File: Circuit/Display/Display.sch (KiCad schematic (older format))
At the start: 29 parts, among them J1 Conn_PIC_ICSP_ICD, J2 Conn_01x04_Female, U1 TBD62783A, U2 PIC16F18854-SO, U3 ULN2803A

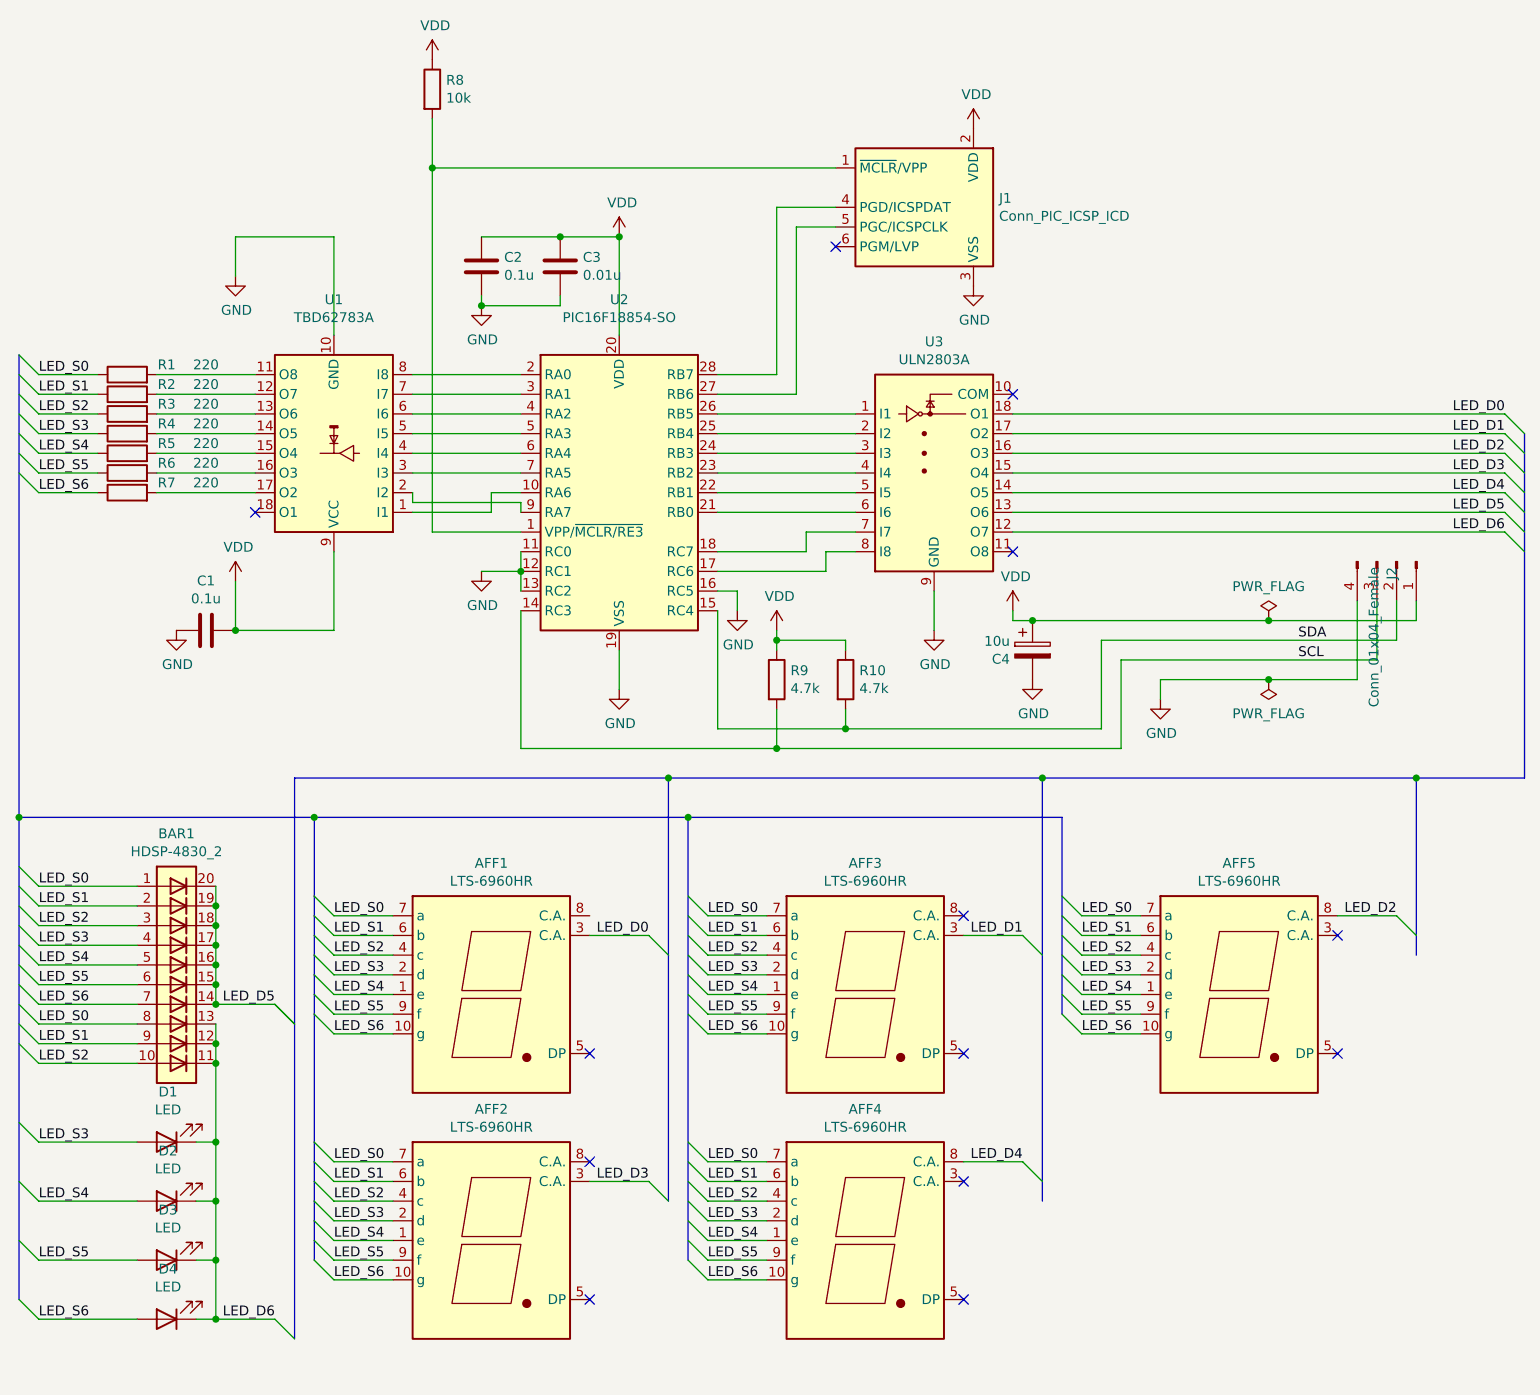
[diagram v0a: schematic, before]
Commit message: 回路完成
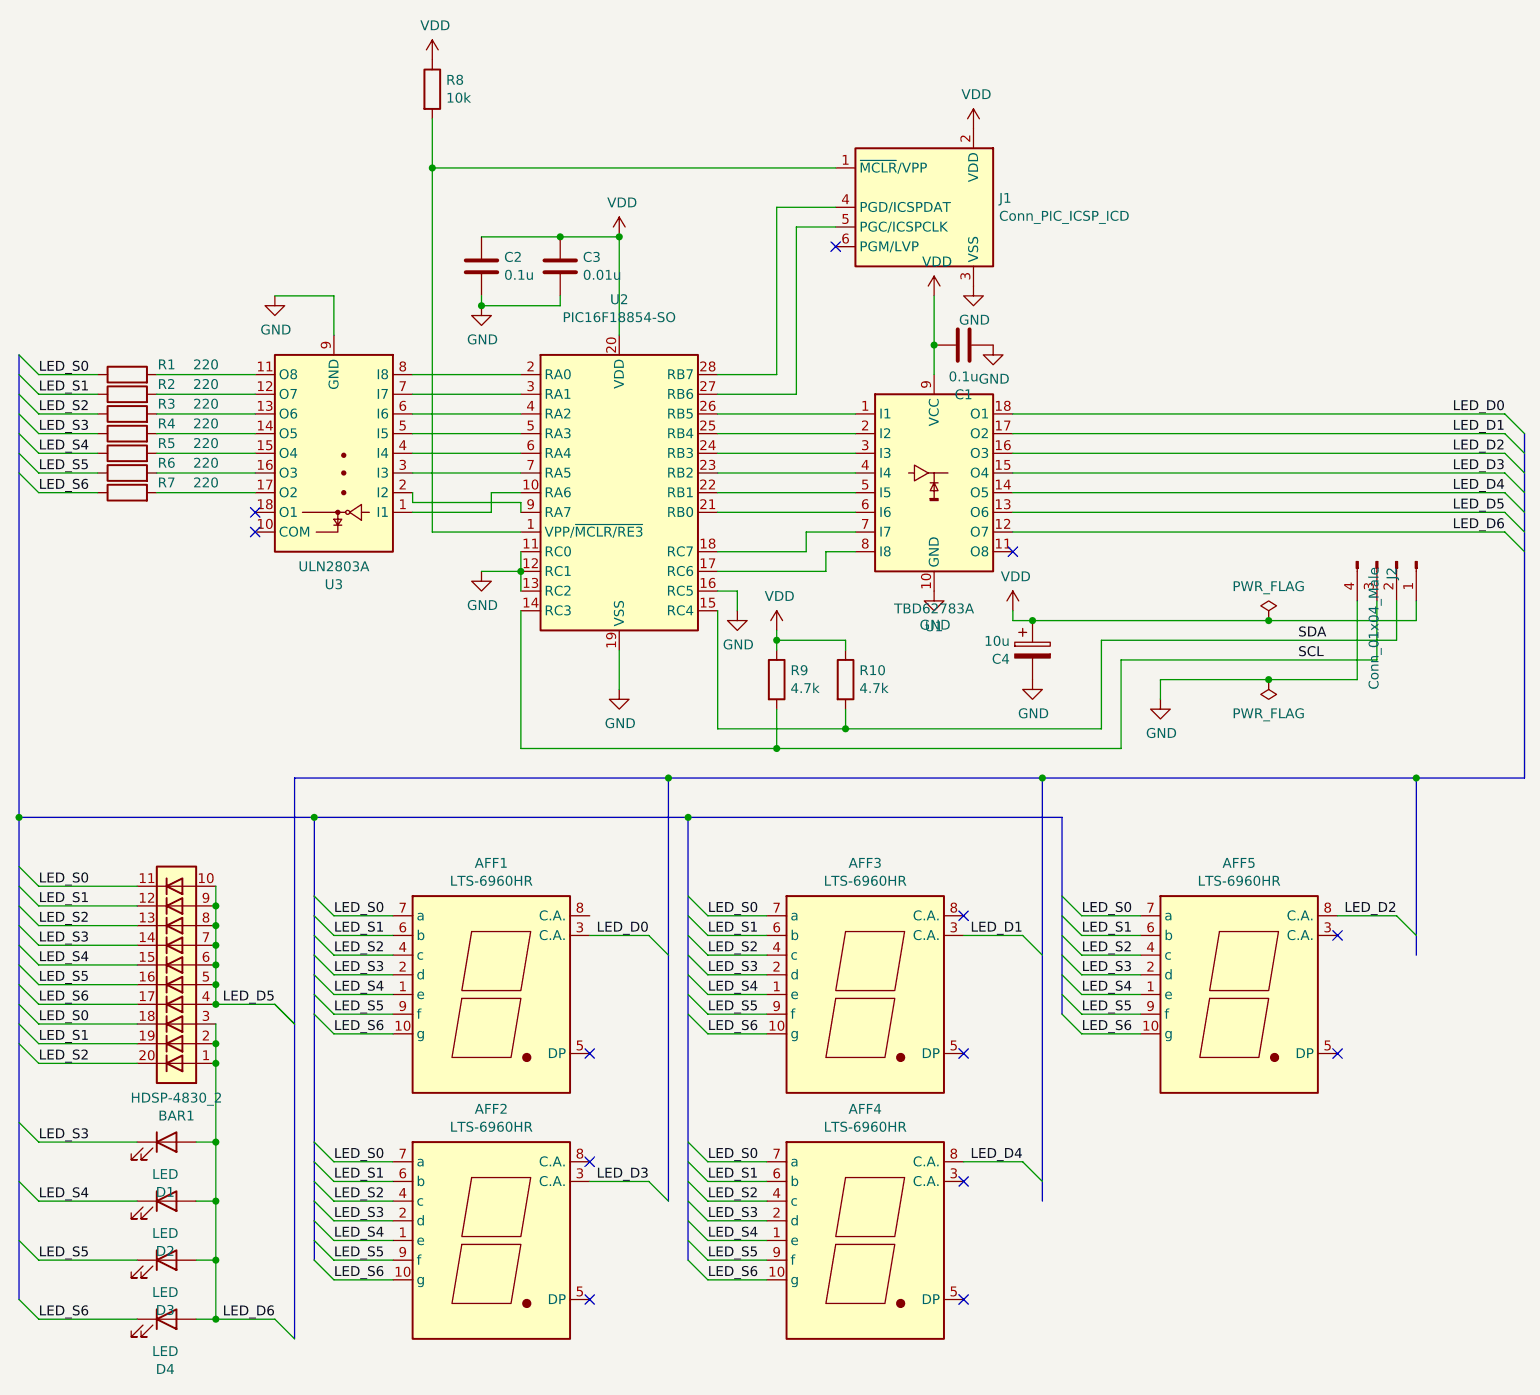
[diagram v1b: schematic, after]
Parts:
- J2: value Conn_01x04_Female -> Conn_01x04_Male
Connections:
- net LED_D0: now also U1.18 (O1); no longer U3.18 (O1)
- net LED_D1: now also U1.17 (O2); no longer U3.17 (O2)
- net LED_D2: now also U1.16 (O3); no longer U3.16 (O3)
- net LED_D3: now also U1.15 (O4); no longer U3.15 (O4)
- net LED_D4: now also U1.14 (O5); no longer U3.14 (O5)
- net LED_D5: now also BAR1.10 (A), BAR1.4 (A), BAR1.5 (A), BAR1.6 (A), BAR1.7 (A), BAR1.8 (A), BAR1.9 (A), U1.13 (O6); no longer BAR1.14 (K), BAR1.15 (K), BAR1.16 (K), BAR1.17 (K), BAR1.18 (K), BAR1.19 (K), BAR1.20 (K), U3.13 (O6)
- net LED_D6: now also BAR1.1 (A), BAR1.2 (A), BAR1.3 (A), D1.2 (A), D2.2 (A), D3.2 (A), D4.2 (A), U1.12 (O7); no longer BAR1.11 (K), BAR1.12 (K), BAR1.13 (K), D1.1 (K), D2.1 (K), D3.1 (K), D4.1 (K), U3.12 (O7)
- net LED_S0: now also BAR1.11 (K), BAR1.18 (K); no longer BAR1.1 (A), BAR1.8 (A)
- net LED_S1: now also BAR1.12 (K), BAR1.19 (K); no longer BAR1.2 (A), BAR1.9 (A)
- net LED_S2: now also BAR1.13 (K), BAR1.20 (K); no longer BAR1.10 (A), BAR1.3 (A)
- net LED_S3: now also BAR1.14 (K), D1.1 (K); no longer BAR1.4 (A), D1.2 (A)
- net LED_S4: now also BAR1.15 (K), D2.1 (K); no longer BAR1.5 (A), D2.2 (A)
- net LED_S5: now also BAR1.16 (K), D3.1 (K); no longer BAR1.6 (A), D3.2 (A)
- net LED_S6: now also BAR1.17 (K), D4.1 (K); no longer BAR1.7 (A), D4.2 (A)
- net at U2.10 (RA6): now also U3.1 (I1); no longer U1.1 (I1)
- net at U2.17 (RC6): now also U1.8 (I8); no longer U3.8 (I8)
- net at U2.18 (RC7): now also U1.7 (I7); no longer U3.7 (I7)
- net at U2.2 (RA0): now also U3.8 (I8); no longer U1.8 (I8)
- net at U2.21 (RB0): now also U1.6 (I6); no longer U3.6 (I6)
- net at U2.22 (RB1): now also U1.5 (I5); no longer U3.5 (I5)
- net at U2.23 (RB2): now also U1.4 (I4); no longer U3.4 (I4)
- net at U2.24 (RB3): now also U1.3 (I3); no longer U3.3 (I3)
- net at U2.25 (RB4): now also U1.2 (I2); no longer U3.2 (I2)
- net at U2.26 (RB5): now also U1.1 (I1); no longer U3.1 (I1)
- net at U2.3 (RA1): now also U3.7 (I7); no longer U1.7 (I7)
- net at U2.4 (RA2): now also U3.6 (I6); no longer U1.6 (I6)
- net at U2.5 (RA3): now also U3.5 (I5); no longer U1.5 (I5)
- net at U2.6 (RA4): now also U3.4 (I4); no longer U1.4 (I4)
- net at U2.7 (RA5): now also U3.3 (I3); no longer U1.3 (I3)
- net at U2.9 (RA7): now also U3.2 (I2); no longer U1.2 (I2)
- net at U1.11 (O8): no longer R1.2
- net at R2.2: now also U3.12 (O7); no longer U1.12 (O7)
- net at R3.2: now also U3.13 (O6); no longer U1.13 (O6)
- net at R4.2: now also U3.14 (O5); no longer U1.14 (O5)
- net at R5.2: now also U3.15 (O4); no longer U1.15 (O4)
- net at R6.2: now also U3.16 (O3); no longer U1.16 (O3)
- net at R7.2: now also U3.17 (O2); no longer U1.17 (O2)
- net at U3.11 (O8): now also R1.2
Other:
- moved on the sheet: C1, D1, D2, D3, D4, U1, U3
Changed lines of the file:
@@
 	4700 5900 5100 5900
 Wire Wire Line
-	4300 4500 3800 4500
-Wire Wire Line
-	4300 5000 4300 4500
-Wire Wire Line
-	4300 6500 4300 6100
-Wire Wire Line
-	3800 6500 4300 6500
+	7350 4800 7350 5050
 $Comp
 L Device:LED D4
@@
 F 3 "~" H 3450 10000 50  0001 C CNN
 	1    3450 10000
-	-1   0    0    1
+	1    0    0    -1
 $EndComp
 $Comp
@@
 F 3 "~" H 3450 9700 50  0001 C CNN
 	1    3450 9700
-	-1   0    0    1
+	1    0    0    -1
 $EndComp
 $Comp
@@
 F 3 "~" H 3450 9400 50  0001 C CNN
 	1    3450 9400
-	-1   0    0    1
+	1    0    0    -1
 $EndComp
 Wire Bus Line
@@
 	4300 7950 4600 7950
 Wire Wire Line
-	3700 8400 4000 8400
-Wire Wire Line
 	4000 10000 3700 10000
 $Comp
@@
 	-1   0    0    1
 $EndComp
-Wire Wire Line
-	3800 6250 3800 6500
 $Comp
 L power:GND #PWR01
 U 1 1 60812496
-P 3500 6500
-F 0 "#PWR01" H 3500 6250 50  0001 C CNN
-F 1 "GND" H 3505 6327 50  0000 C CNN
-F 2 "" H 3500 6500 50  0001 C CNN
-F 3 "" H 3500 6500 50  0001 C CNN
-	1    3500 6500
-	1    0    0    -1
-$EndComp
-Connection ~ 3800 6500
+P 7650 5050
+F 0 "#PWR01" H 7650 4800 50  0001 C CNN
+F 1 "GND" H 7655 4877 50  0000 C CNN
+F 2 "" H 7650 5050 50  0001 C CNN
+F 3 "" H 7650 5050 50  0001 C CNN
+	1    7650 5050
+	1    0    0    -1
+$EndComp
 $Comp
 L Device:C C1
 U 1 1 60811A21
-P 3650 6500
-F 0 "C1" V 3398 6500 50  0000 C CNN
-F 1 "0.1u" V 3489 6500 50  0000 C CNN
-F 2 "Capacitor_THT:C_Disc_D3.0mm_W1.6mm_P2.50mm" H 3688 6350 50  0001 C CNN
-F 3 "~" H 3650 6500 50  0001 C CNN
-	1    3650 6500
-	0    1    1    0
+P 7500 5050
+F 0 "C1" V 7248 5050 50  0000 C CNN
+F 1 "0.1u" V 7339 5050 50  0000 C CNN
+F 2 "Capacitor_THT:C_Disc_D3.0mm_W1.6mm_P2.50mm" H 7538 4900 50  0001 C CNN
+F 3 "~" H 7500 5050 50  0001 C CNN
+	1    7500 5050
+	0    -1   -1   0
 $EndComp
 Connection ~ 5750 4500
@@
 L power:VDD #PWR02
 U 1 1 607FC6E4
-P 3800 6250
-F 0 "#PWR02" H 3800 6100 50  0001 C CNN
-F 1 "VDD" H 3815 6423 50  0000 C CNN
-F 2 "" H 3800 6250 50  0001 C CNN
-F 3 "" H 3800 6250 50  0001 C CNN
-	1    3800 6250
+P 7350 4800
+F 0 "#PWR02" H 7350 4650 50  0001 C CNN
+F 1 "VDD" H 7365 4973 50  0000 C CNN
+F 2 "" H 7350 4800 50  0001 C CNN
+F 3 "" H 7350 4800 50  0001 C CNN
+	1    7350 4800
 	1    0    0    -1
 $EndComp
@@
 	1    0    0    -1
 $EndComp
-NoConn ~ 7750 5300
 NoConn ~ 7750 6100
 NoConn ~ 3900 5900
@@
 Wire Wire Line
 	3700 9100 3700 9400
-Connection ~ 3700 9100
 Wire Wire Line
 	3600 9100 3700 9100
@@
 LED_S0
 Wire Wire Line
-	3300 8400 2800 8400
-Wire Wire Line
 	2800 8300 3300 8300
 Wire Wire Line
@@
 Wire Wire Line
 	2800 8100 3300 8100
-Wire Wire Line
-	3300 8000 2800 8000
 Wire Wire Line
 	2800 7900 3300 7900
@@
 L Transistor_Array:ULN2803A U3
 U 1 1 6035D1F1
-P 7350 5600
-F 0 "U3" H 7350 6167 50  0000 C CNN
-F 1 "ULN2803A" H 7350 6076 50  0000 C CNN
-F 2 "Package_DIP:DIP-18_W7.62mm" H 7400 4950 50  0001 L CNN
-F 3 "http://www.ti.com/lit/ds/symlink/uln2803a.pdf" H 7450 5400 50  0001 C CNN
-	1    7350 5600
-	1    0    0    -1
+P 4300 5700
+F 0 "U3" H 4300 6267 50  0000 C CNN
+F 1 "ULN2803A" H 4300 6176 50  0000 C CNN
+F 2 "Package_DIP:DIP-18_W7.62mm" H 4350 5050 50  0001 L CNN
+F 3 "http://www.ti.com/lit/ds/symlink/uln2803a.pdf" H 4400 5500 50  0001 C CNN
+	1    4300 5700
+	-1   0    0    1
 $EndComp
 $Comp
 L Transistor_Array:TBD62783A U1
 U 1 1 60340DE8
-P 4300 5600
-F 0 "U1" H 4300 4819 50  0000 C CNN
-F 1 "TBD62783A" H 4300 4910 50  0000 C CNN
-F 2 "Package_DIP:DIP-18_W7.62mm" H 4300 5050 50  0001 C CNN
-F 3 "http://toshiba.semicon-storage.com/info/docget.jsp?did=30523&prodName=TBD62783APG" H 4000 6000 50  0001 C CNN
-	1    4300 5600
-	-1   0    0    1
-$EndComp
-Wire Wire Line
-	3700 7800 3700 7900
-Connection ~ 3700 7900
-Wire Wire Line
-	3700 7900 3700 8000
-Connection ~ 3700 8000
-Wire Wire Line
-	3700 8000 3700 8100
-Connection ~ 3700 8100
-Wire Wire Line
-	3700 8100 3700 8200
-Connection ~ 3700 8200
-Wire Wire Line
-	3700 8300 3700 8400
-Wire Wire Line
-	3700 8200 3700 8300
-Connection ~ 3700 8300
-Connection ~ 3700 8400
-Wire Wire Line
-	3700 8500 3700 8600
-Connection ~ 3700 8600
-Wire Wire Line
-	3700 9100 3700 8700
-Wire Wire Line
-	3700 8600 3700 8700
-Connection ~ 3700 8700
-$Comp
-L LED:HDSP-4830_2 BAR1
-U 1 1 60332800
-P 3500 8200
-F 0 "BAR1" H 3500 8867 50  0000 C CNN
-F 1 "HDSP-4830_2" H 3500 8776 50  0000 C CNN
-F 2 "Display:HDSP-4830" H 3500 7400 50  0001 C CNN
-F 3 "https://docs.broadcom.com/docs/AV02-1798EN" H 1500 8400 50  0001 C CNN
-	1    3500 8200
+P 7350 5700
+F 0 "U1" H 7350 4919 50  0000 C CNN
+F 1 "TBD62783A" H 7350 5010 50  0000 C CNN
+F 2 "Package_DIP:DIP-18_W7.62mm" H 7350 5150 50  0001 C CNN
+F 3 "http://toshiba.semicon-storage.com/info/docget.jsp?did=30523&prodName=TBD62783APG" H 7050 6100 50  0001 C CNN
+	1    7350 5700
 	1    0    0    -1
 $EndComp
@@
 F 3 "~" H 3450 9100 50  0001 C CNN
 	1    3450 9100
-	-1   0    0    1
+	1    0    0    -1
 $EndComp
 Wire Wire Line
@@
 $EndComp
 Wire Wire Line
-	7350 6300 7350 6500
+	4300 5000 4300 4800
 $Comp
 L power:GND #PWR09
 U 1 1 602E59D5
-P 7350 6500
-F 0 "#PWR09" H 7350 6250 50  0001 C CNN
-F 1 "GND" H 7355 6327 50  0000 C CNN
-F 2 "" H 7350 6500 50  0001 C CNN
-F 3 "" H 7350 6500 50  0001 C CNN
-	1    7350 6500
+P 4000 4800
+F 0 "#PWR09" H 4000 4550 50  0001 C CNN
+F 1 "GND" H 4005 4627 50  0000 C CNN
+F 2 "" H 4000 4800 50  0001 C CNN
+F 3 "" H 4000 4800 50  0001 C CNN
+	1    4000 4800
 	1    0    0    -1
 $EndComp
@@
 	1    0    0    -1
 $EndComp
-Wire Wire Line
-	3800 4500 3800 4700
 $Comp
 L power:GND #PWR03
 U 1 1 602E0BCF
-P 3800 4700
-F 0 "#PWR03" H 3800 4450 50  0001 C CNN
-F 1 "GND" H 3805 4527 50  0000 C CNN
-F 2 "" H 3800 4700 50  0001 C CNN
-F 3 "" H 3800 4700 50  0001 C CNN
-	1    3800 4700
+P 7350 6300
+F 0 "#PWR03" H 7350 6050 50  0001 C CNN
+F 1 "GND" H 7355 6127 50  0000 C CNN
+F 2 "" H 7350 6300 50  0001 C CNN
+F 3 "" H 7350 6300 50  0001 C CNN
+	1    7350 6300
 	1    0    0    -1
 $EndComp
@@
 P 9700 6150
 F 0 "J2" H 9728 6126 50  0000 L CNN
-F 1 "Conn_01x04_Female" H 9728 6035 50  0000 L CNN
+F 1 "Conn_01x04_Male" H 9728 6035 50  0000 L CNN
 F 2 "Connector_PinHeader_2.54mm:PinHeader_1x04_P2.54mm_Horizontal" H 9700 6150 50  0001 C CNN
 F 3 "~" H 9700 6150 50  0001 C CNN
@@
 	0    1    1    0
 $EndComp
-Wire Bus Line
-	4100 7250 4100 10100
-Wire Bus Line
-	6000 7250 6000 9400
-Wire Bus Line
-	9800 7250 9800 8150
-Wire Bus Line
-	7900 7250 7900 9400
-Wire Bus Line
-	8000 7450 8000 8450
-Wire Bus Line
-	10350 5500 10350 7250
-Wire Bus Line
-	2700 5100 2700 7450
-Wire Bus Line
-	6100 7450 6100 9700
-Wire Bus Line
-	2700 7450 2700 9900
-Wire Bus Line
-	4200 7450 4200 9700
 Text Label 9200 6550 0    50   ~ 0
 SDA
 Text Label 9200 6650 0    50   ~ 0
 SCL
+Connection ~ 3700 8000
+Connection ~ 3700 9100
+Connection ~ 3700 8700
+Wire Wire Line
+	3700 9100 3700 8700
+Connection ~ 3700 8600
+Wire Wire Line
+	3700 8600 3700 8700
+Wire Wire Line
+	3700 8500 3700 8600
+Connection ~ 3700 8400
+Connection ~ 3700 8300
+Wire Wire Line
+	3700 8200 3700 8300
+Wire Wire Line
+	3700 8300 3700 8400
+Connection ~ 3700 8200
+Connection ~ 3700 8100
+Wire Wire Line
+	3700 8100 3700 8200
+Wire Wire Line
+	3700 8000 3700 8100
+Connection ~ 3700 7900
+Wire Wire Line
+	3700 7900 3700 8000
+Wire Wire Line
+	3700 7800 3700 7900
+Wire Wire Line
+	3700 8400 4000 8400
+Wire Wire Line
+	3300 8400 2800 8400
+Wire Wire Line
+	3300 8000 2800 8000
+$Comp
+L LED:HDSP-4830_2 BAR1
+U 1 1 60332800
+P 3500 8300
+F 0 "BAR1" H 3500 8967 50  0000 C CNN
+F 1 "HDSP-4830_2" H 3500 8876 50  0000 C CNN
+F 2 "Display:HDSP-4830" H 3500 7500 50  0001 C CNN
+F 3 "https://docs.broadcom.com/docs/AV02-1798EN" H 1500 8500 50  0001 C CNN
+	1    3500 8300
+	-1   0    0    1
+$EndComp
+NoConn ~ 3900 6000
+Wire Wire Line
+	4000 4800 4300 4800
+Wire Bus Line
+	4100 7250 4100 10100
+Wire Bus Line
+	6000 7250 6000 9400
+Wire Bus Line
+	9800 7250 9800 8150
+Wire Bus Line
+	7900 7250 7900 9400
+Wire Bus Line
+	8000 7450 8000 8450
+Wire Bus Line
+	10350 5500 10350 7250
+Wire Bus Line
+	2700 5100 2700 7450
+Wire Bus Line
+	6100 7450 6100 9700
+Wire Bus Line
+	2700 7450 2700 9900
+Wire Bus Line
+	4200 7450 4200 9700
+Connection ~ 7350 5050
+Wire Wire Line
+	7350 5050 7350 5200
 $EndSCHEMATC
